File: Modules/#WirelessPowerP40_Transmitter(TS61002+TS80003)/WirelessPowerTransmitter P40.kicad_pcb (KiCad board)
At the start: 4 copper layers, 53 x 49 mm, 119 parts, among them J1 USBA, J2 I2C, J3 I2C, J4 Coil Therm, J5 COIL 20uH, U1 TS30041, U2 TS94033, U3 74LVC1G66, U4 TS61002, U5 TS80003, U6 BSC0993ND, U7 BSC0993ND

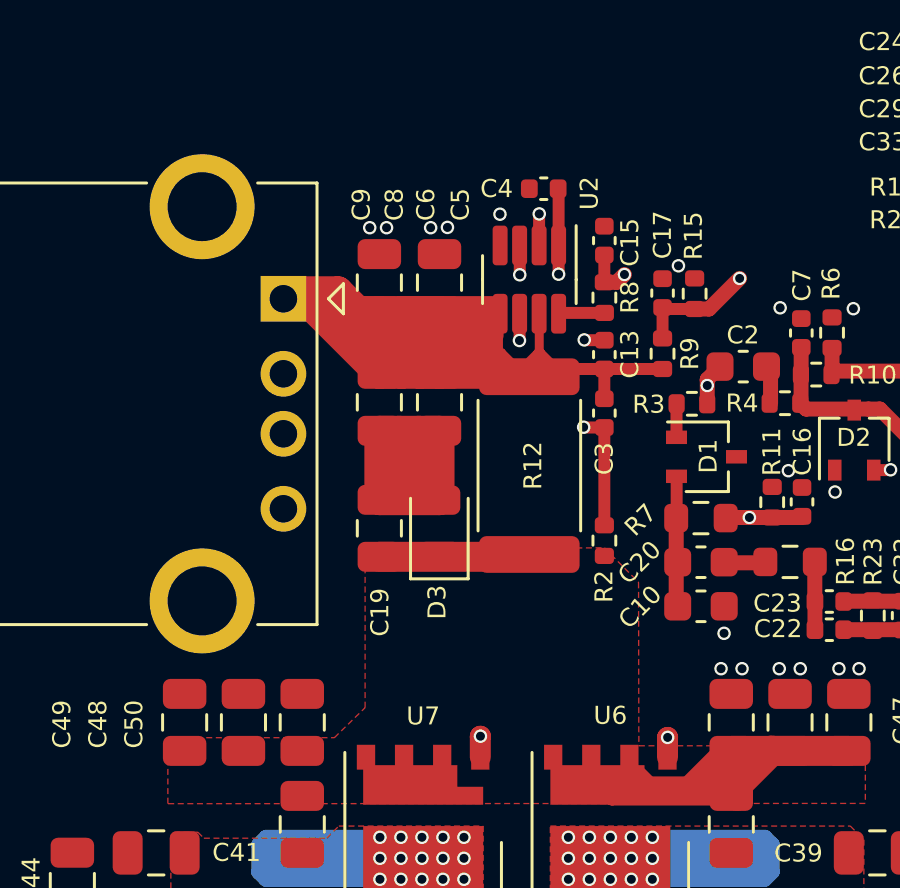
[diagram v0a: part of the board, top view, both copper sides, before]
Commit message: WirelessPowerP40_Transmitter update
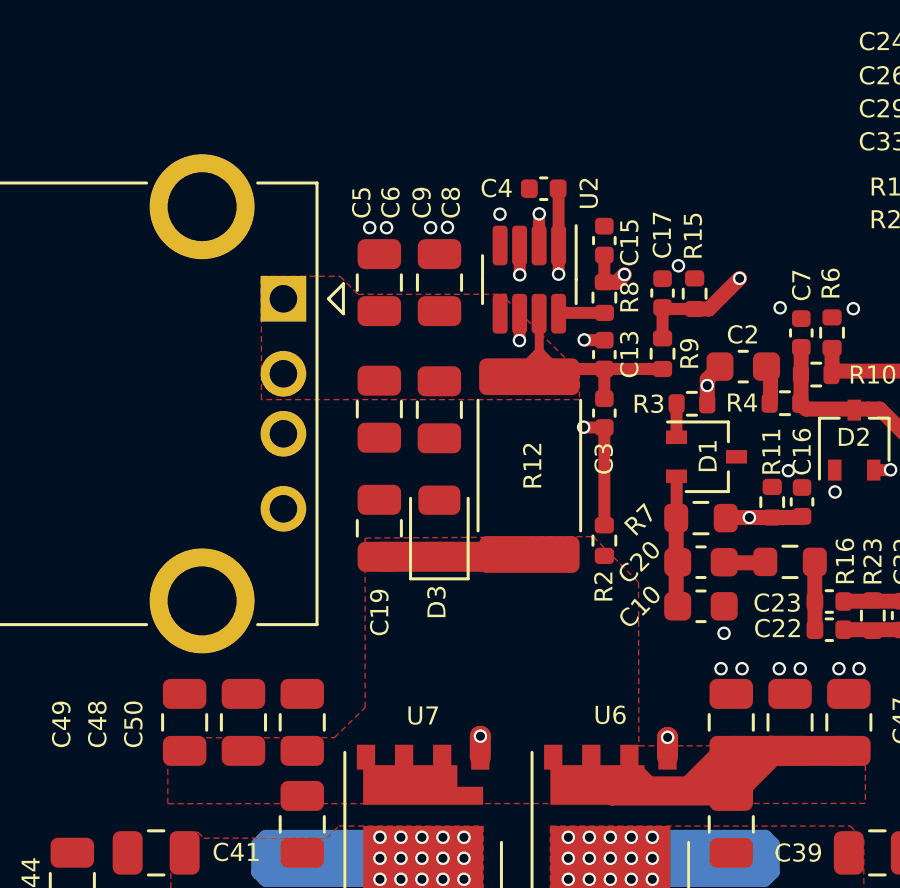
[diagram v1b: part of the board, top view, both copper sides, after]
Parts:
- moved C9 2.02 mm to (124.0, 89.5)
- moved C8 2.02 mm to (126.0, 89.5)
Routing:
- net DC_I+: track 139.8 -> 106.3 mm
- net GND: track 48.7 -> 35.5 mm
- added copper zone on F.Cu, net DC_I+
